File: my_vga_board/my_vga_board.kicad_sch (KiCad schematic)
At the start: 30 parts, among them J1 Barrel_Jack, J2 L77HDE15SD1CH4F, J3 I2C_A, J4 I2C_B, U1 Pico, U2 LM7805_TO220

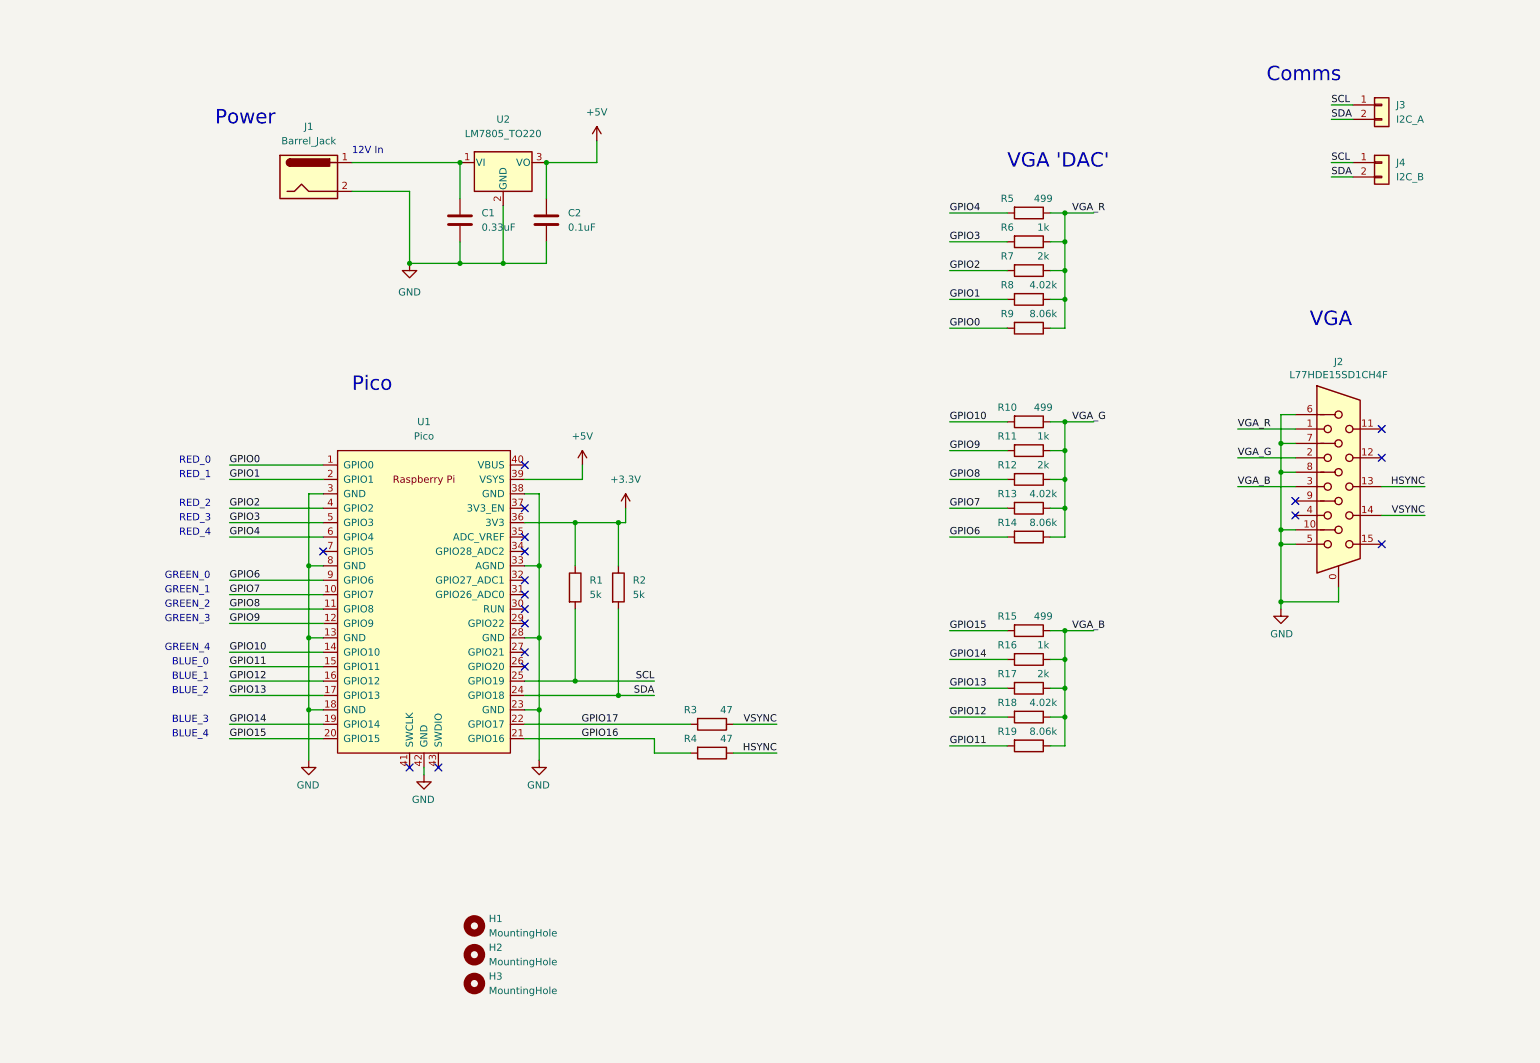
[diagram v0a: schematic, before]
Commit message: R-2R
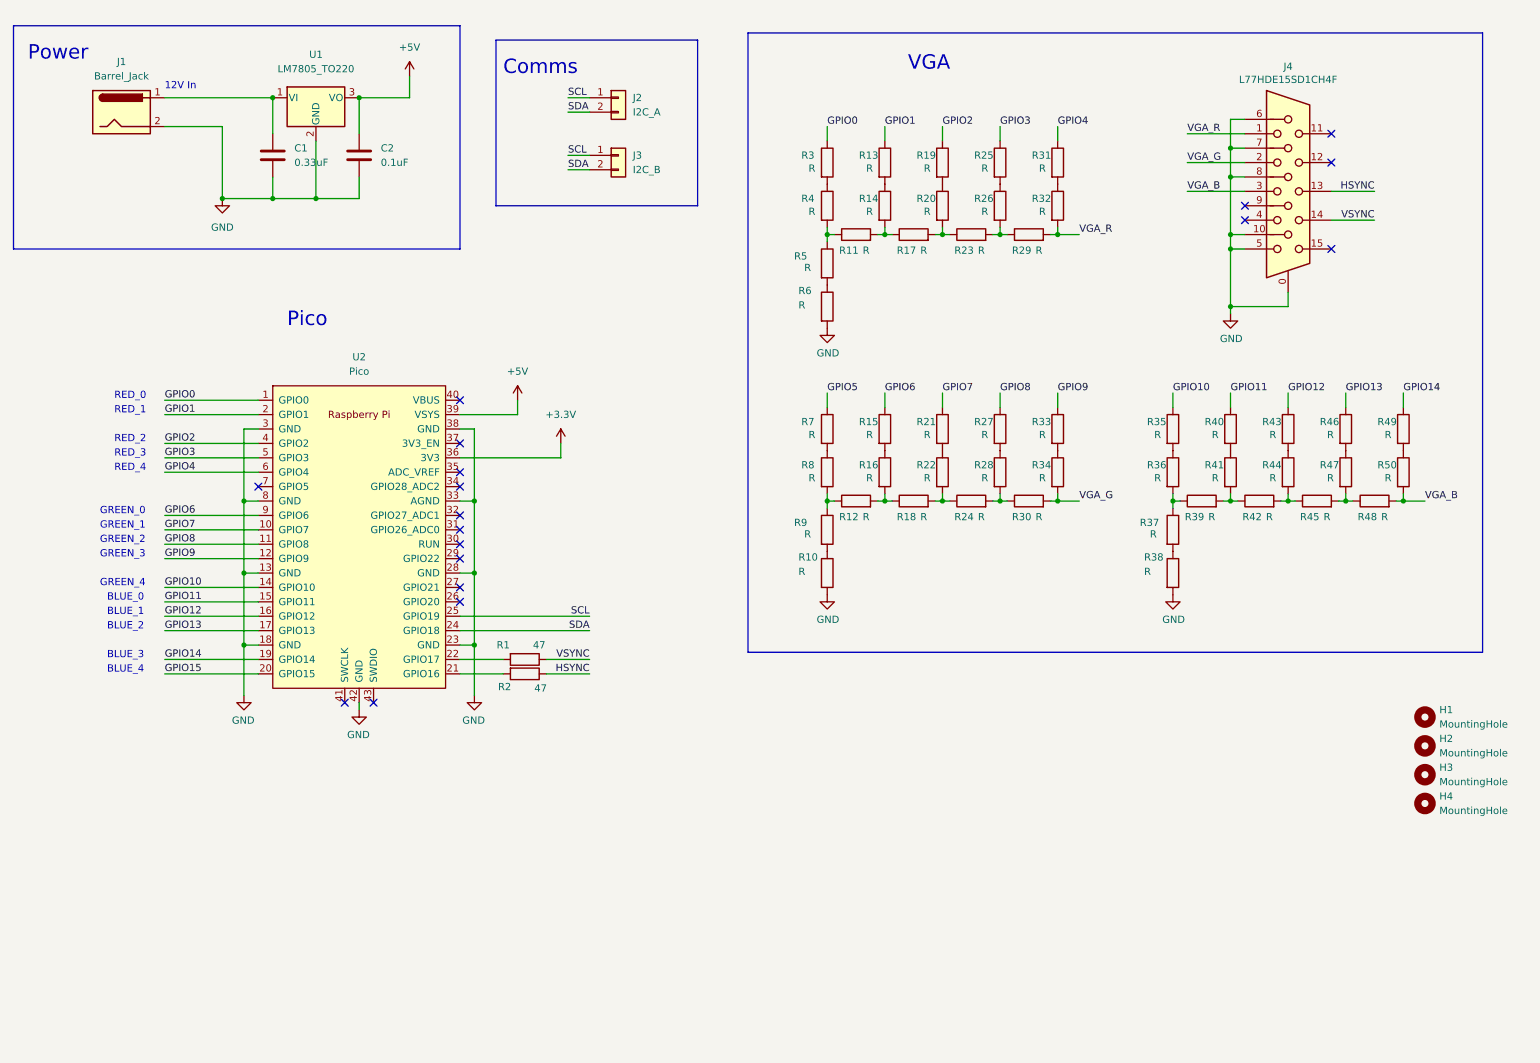
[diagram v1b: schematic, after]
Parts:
- removed R1, R2: 5k, Resistor_THT:R_Axial_DIN0207_L6.3mm_D2.5mm_P7.62mm_Horizontal, symbol Device:R
- added H4: MountingHole, MountingHole:MountingHole_4.3mm_M4, symbol Mechanical:MountingHole
- added R20, R21, R22, R23, R24, R25, R26, R27, R28, R29, R3, R30, R31, R32, R33, R34, R35, R36, R37, R38, R39, R4, R40, R41, R42, R43, R44, R45, R46, R47, R48, R49, R50: R, Resistor_SMD:R_0603_1608Metric_Pad0.98x0.95mm_HandSolder, symbol Device:R
- R1: renamed from R3; footprint Resistor_THT:R_Axial_DIN0207_L6.3mm_D2.5mm_P7.62mm_Horizontal -> Resistor_SMD:R_0603_1608Metric_Pad0.98x0.95mm_HandSolder
- R10, R15, R5: value 499 -> R; footprint Resistor_THT:R_Axial_DIN0207_L6.3mm_D2.5mm_P7.62mm_Horizontal -> Resistor_SMD:R_0603_1608Metric_Pad0.98x0.95mm_HandSolder
- R11, R16, R6: value 1k -> R; footprint Resistor_THT:R_Axial_DIN0207_L6.3mm_D2.5mm_P7.62mm_Horizontal -> Resistor_SMD:R_0603_1608Metric_Pad0.98x0.95mm_HandSolder
- R12, R17, R7: value 2k -> R; footprint Resistor_THT:R_Axial_DIN0207_L6.3mm_D2.5mm_P7.62mm_Horizontal -> Resistor_SMD:R_0603_1608Metric_Pad0.98x0.95mm_HandSolder
- R13, R18, R8: value 4.02k -> R; footprint Resistor_THT:R_Axial_DIN0207_L6.3mm_D2.5mm_P7.62mm_Horizontal -> Resistor_SMD:R_0603_1608Metric_Pad0.98x0.95mm_HandSolder
- R14, R19, R9: value 8.06k -> R; footprint Resistor_THT:R_Axial_DIN0207_L6.3mm_D2.5mm_P7.62mm_Horizontal -> Resistor_SMD:R_0603_1608Metric_Pad0.98x0.95mm_HandSolder
- R2: renamed from R4; footprint Resistor_THT:R_Axial_DIN0207_L6.3mm_D2.5mm_P7.62mm_Horizontal -> Resistor_SMD:R_0603_1608Metric_Pad0.98x0.95mm_HandSolder
- renumbered J3 to J2, J4 to J3, J2 to J4, U2 to U1, U1 to U2
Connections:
- net GND: now also R10.2, R6.2, R38.2
- net GPIO0: now also R3.1; no longer R9.2
- net GPIO1: now also R13.1; no longer R8.2
- net GPIO10: now also R35.1; no longer R10.2
- net GPIO11: now also R40.1; no longer R19.2
- net GPIO12: now also R43.1; no longer R18.2
- net GPIO13: now also R46.1; no longer R17.2
- net GPIO14: now also R49.1; no longer R16.2
- net GPIO15: no longer R15.2
- net GPIO2: now also R19.1; no longer R7.2
- net GPIO3: now also R25.1; no longer R6.2
- net GPIO4: now also R31.1; no longer R5.2
- net GPIO6: now also R15.1; no longer R14.2
- net GPIO7: now also R21.1; no longer R13.2
- net GPIO8: now also R27.1; no longer R12.2
- net GPIO9: now also R33.1; no longer R11.2
- net VGA_B: now also R48.2, R50.2; no longer R15.1, R16.1, R17.1, R18.1, R19.1
- net VGA_G: now also R30.2, R34.2; no longer R10.1, R11.1, R12.1, R13.1, R14.1
- net VGA_R: now also R29.2, R32.2; no longer R5.1, R6.1, R7.1, R8.1, R9.1
- net GPIO16: no longer names the net of R2.2, U2.21 (GPIO16)
- net GPIO17: no longer names the net of R1.2, U2.22 (GPIO17)
- new net: R12.2, R16.2, R18.1
- new net: R18.2, R22.2, R24.1
- new net: R35.2, R36.1
- new net: R36.2, R37.1, R39.1
- new net: R17.2, R20.2, R23.1
- new net: R23.2, R26.2, R29.1
- new net: R3.2, R4.1
- new net: R11.1, R4.2, R5.1
- new net: R5.2, R6.1
- new net: R37.2, R38.1
- new net: R11.2, R14.2, R17.1
- new net: R40.2, R41.1
- new net: R39.2, R41.2, R42.1
- new net: R15.2, R16.1
- new net: R46.2, R47.1
- new net: R49.2, R50.1
- new net: R31.2, R32.1
- new net: R45.2, R47.2, R48.1
- new net: R42.2, R44.2, R45.1
- new net: R21.2, R22.1
- new net: R19.2, R20.1
- new net: R13.2, R14.1
- new net: R12.1, R8.2, R9.1
- new net: R10.1, R9.2
- new net: R43.2, R44.1
- new net: R27.2, R28.1
- new net: R33.2, R34.1
- new net: R24.2, R28.2, R30.1
- new net: R7.2, R8.1
- new net: R25.2, R26.1
- new net GPIO5: R7.1
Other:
- note removed: "VGA 'DAC'"
- moved on the sheet: C1, C2, H1, H2, H3, J1, J2, J3, J4, R1, R2, U1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

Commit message: some sound
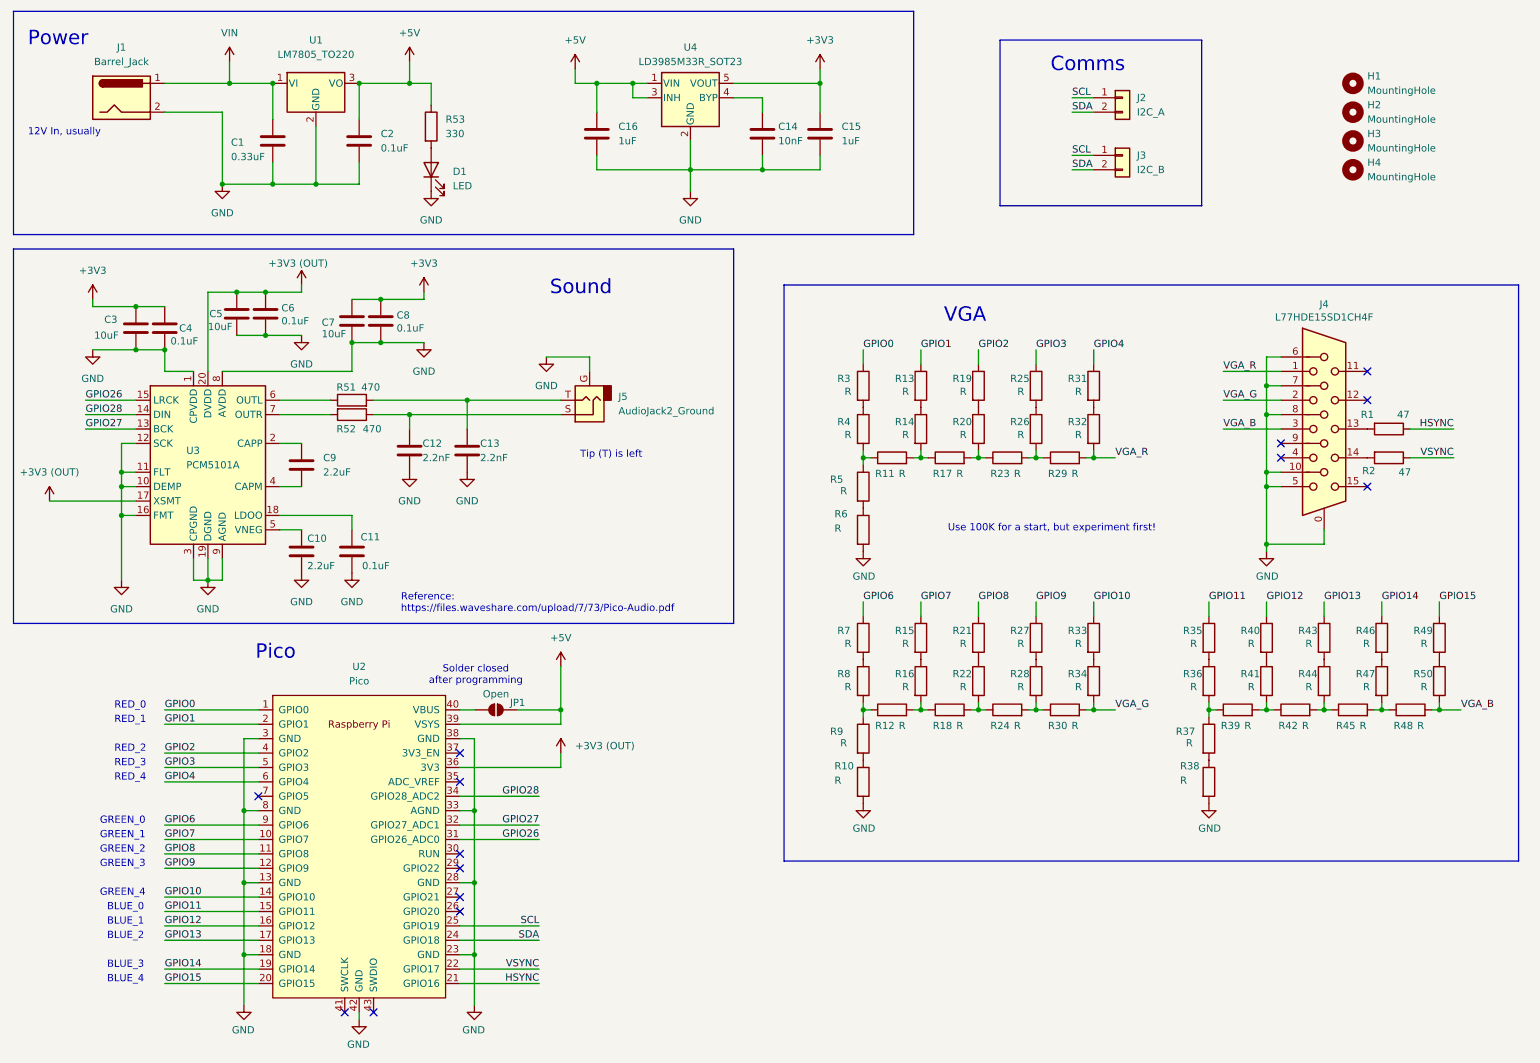
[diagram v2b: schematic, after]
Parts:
- added C10, C9: 2.2uF, symbol Device:C
- added C11, C4, C6, C8: 0.1uF, symbol Device:C
- added C12, C13: 2.2nF, symbol Device:C
- added C14: 10nF, symbol Device:C
- added C15, C16: 1uF, symbol Device:C
- added C3, C5, C7: 10uF, symbol Device:C
- added D1: LED, LED_THT:LED_D5.0mm, symbol Device:LED
- added J5: AudioJack2_Ground, Connector_Audio:Jack_3.5mm_CUI_SJ1-3533NG_Horizontal, symbol Connector_Audio:AudioJack2_Ground
- added JP1: Open, Jumper:SolderJumper-2_P1.3mm_Open_Pad1.0x1.5mm, symbol Jumper:SolderJumper_2_Open
- added R51, R52: 470, Resistor_SMD:R_0603_1608Metric_Pad0.98x0.95mm_HandSolder, symbol Device:R
- added R53: 330, Resistor_THT:R_Axial_DIN0207_L6.3mm_D2.5mm_P7.62mm_Horizontal, symbol Device:R
- added U3: PCM5101A, Package_SO:TSSOP-20_4.4x6.5mm_P0.65mm, symbol Audio:PCM5101A
- added U4: LD3985M33R_SOT23, Package_TO_SOT_SMD:SOT-23-5, symbol Regulator_Linear:LD3985M33R_SOT23
- U1: footprint Package_TO_SOT_THT:TO-220-3_Vertical -> Package_TO_SOT_THT:TO-220-3_Horizontal_TabDown
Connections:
- net GPIO5 is gone; now on net GPIO6: R7.1
- net +5V: now also C16.1, JP1.2 (B), R53.1, U4.1 (VIN), U4.3 (INH)
- net GND: now also C10.2, C11.2, C12.2, C13.2, C14.2, C15.2, C16.2, C3.2, C4.2, C5.2, C6.2, C7.2, C8.2, D1.1 (K), J5.G, U3.1 (CPVDD), U3.10 (DEMP), U3.11 (FLT), U3.12 (SCK), U3.16 (FMT), U3.19 (DGND), U3.3 (CPGND), U3.8 (AVDD), U3.9 (AGND), U4.2 (GND)
- net GPIO10: now also R33.1; no longer R35.1
- net GPIO11: now also R35.1; no longer R40.1
- net GPIO12: now also R40.1; no longer R43.1
- net GPIO13: now also R43.1; no longer R46.1
- net GPIO14: now also R46.1; no longer R49.1
- net GPIO15: now also R49.1
- net GPIO6: no longer R15.1
- net GPIO7: now also R15.1; no longer R21.1
- net GPIO8: now also R21.1; no longer R27.1
- net GPIO9: now also R27.1; no longer R33.1
- net HSYNC: now also R1.1, U2.21 (GPIO16); no longer J4.13, R2.1
- net VSYNC: now also R2.1, U2.22 (GPIO17); no longer J4.14, R1.1
- net at R1.2: now also J4.13; no longer U2.22 (GPIO17)
- net at R2.2: now also J4.14; no longer U2.21 (GPIO16)
- net VIN: now reaches C1.1, J1.1, U1.1 (VI)
- net GPIO26: now reaches U2.31 (GPIO26_ADC0)
- net GPIO26: now also U3.15 (LRCK)
- net GPIO27: now reaches U2.32 (GPIO27_ADC1)
- net GPIO27: now also U3.13 (BCK)
- net GPIO28: now reaches U2.34 (GPIO28_ADC2)
- net GPIO28: now also U3.14 (DIN)
- net at U2.40 (VBUS): now also JP1.1 (A)
- net +3.3V renamed +3V3 (OUT)
- net +3V3 (OUT): now also C5.1, C6.1, U3.17 (XSMT), U3.20 (DVDD)
- new net: C11.1, U3.18 (LDOO)
- new net: C9.1, U3.2 (CAPP)
- new net: C9.2, U3.4 (CAPM)
- new net: C10.1, U3.5 (VNEG)
- new net: R51.1, U3.6 (OUTL)
- new net: R52.2, U3.7 (OUTR)
- new net: C14.1, U4.4 (BYP)
- new net: C12.1, J5.S, R52.1
- new net: D1.2 (A), R53.2
- new net: C13.1, J5.T, R51.2
- new net +3V3: C15.1, C3.1, C4.1, C7.1, C8.1, U4.5 (VOUT)
- no-connect marks 18 -> 14
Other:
- note added: "12V In, usually"
- note added: "Reference: https://files.waveshare.com/upload/7/73/Pico-Audio.pdf"
- note added: "Solder closed after programming"
- note added: "Sound"
- note added: "Tip (T) is left"
- note added: "Use 100K for a start, but experiment first!"
- note removed: "12V In"
- moved on the sheet: C1, C2, H1, H2, H3, H4, J1, J2, J3, J4, R1, R10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
